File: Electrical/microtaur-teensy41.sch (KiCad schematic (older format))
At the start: 32 parts, among them J2 USB_A, U1 Teensy4.1, U3 LM7805_TO220

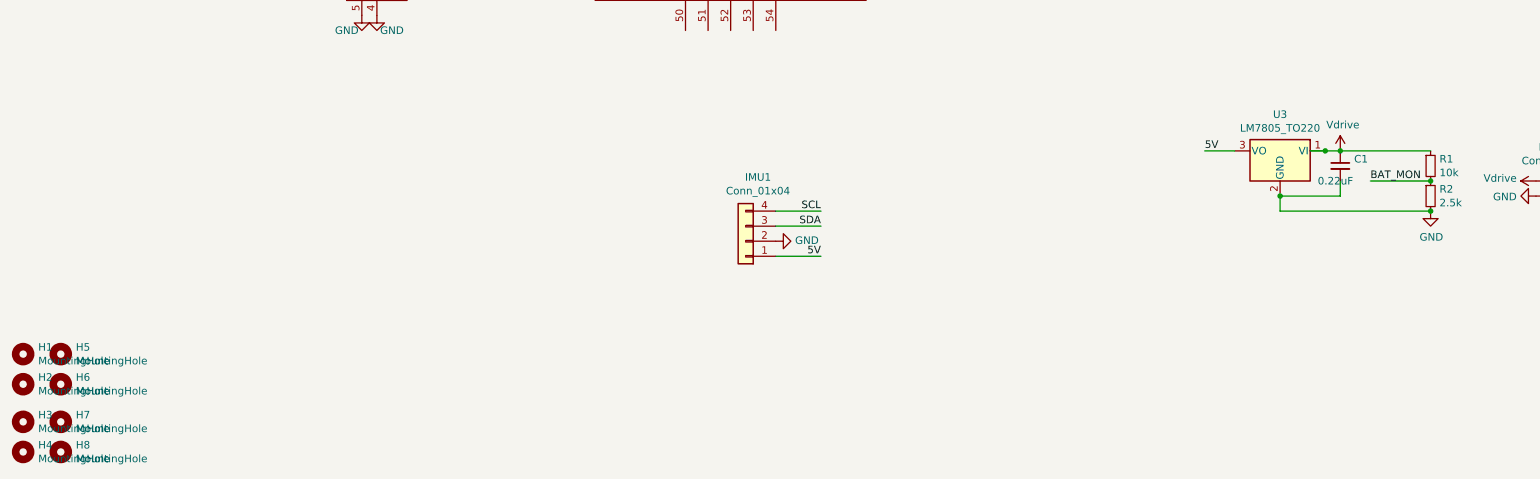
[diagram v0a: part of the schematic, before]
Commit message: completed pcb design, ready to fab
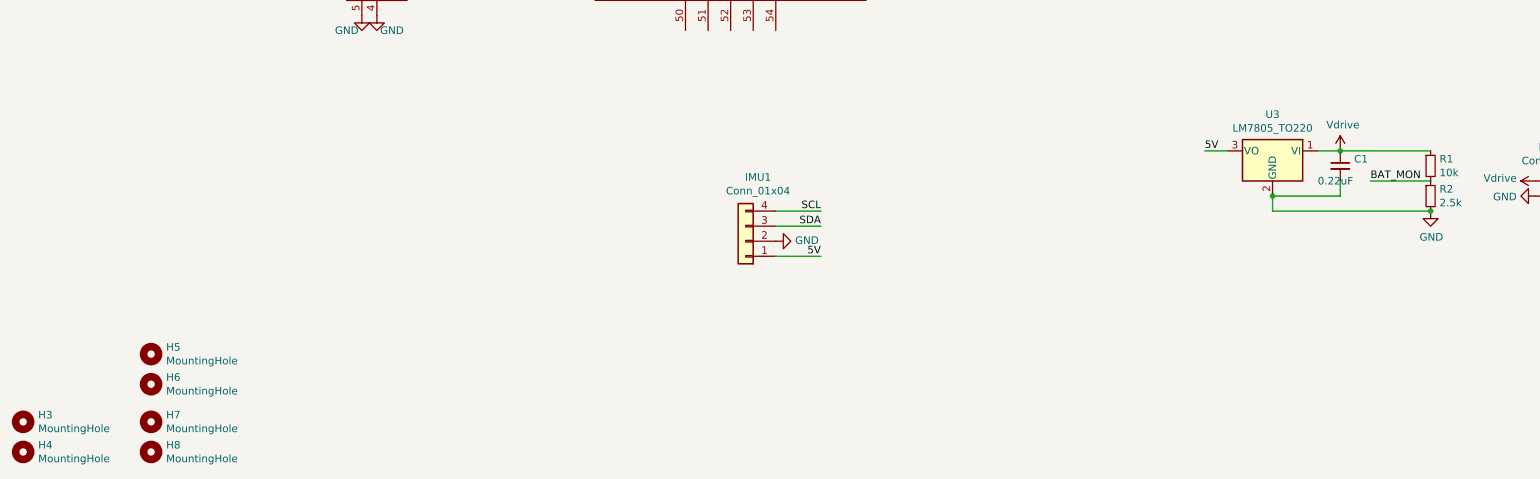
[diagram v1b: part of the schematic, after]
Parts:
- removed H1, H2: MountingHole, MountingHole:MountingHole_2.2mm_M2, symbol Mechanical:MountingHole
- IMU1: footprint Connector_JST:JST_SH_BM04B-SRSS-TB_1x04-1MP_P1.00mm_Vertical -> Connector_JST:JST_SH_SM04B-SRSS-TB_1x04-1MP_P1.00mm_Horizontal
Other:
- moved on the sheet: H5, H6, H7, H8, U3
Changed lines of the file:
@@
 Wire Wire Line
 	10100 5650 9700 5650
-Connection ~ 10100 5650
 Text Label 9700 5650 0    50   ~ 0
 BAT_MON
@@
 Text Label 6050 6150 2    50   ~ 0
 5V
-Connection ~ 9500 5450
 $Comp
 L Device:C_Small C1
@@
 $EndComp
 Wire Wire Line
-	9100 5750 9500 5750
+	9050 5750 9500 5750
 Wire Wire Line
 	9500 5750 9500 5650
 Wire Wire Line
-	9100 5850 9100 5750
-Wire Wire Line
-	9500 5450 10100 5450
-Wire Wire Line
-	9100 5850 10100 5850
-Connection ~ 10100 5850
-Wire Wire Line
-	8600 5450 8800 5450
+	9050 5850 9050 5750
+Wire Wire Line
+	9050 5850 10100 5850
 Text Label 8600 5450 0    50   ~ 0
 5V
@@
 L Mechanical:MountingHole H7
 U 1 1 608B8276
-P 1000 7250
-F 0 "H7" H 1100 7296 50  0000 L CNN
-F 1 "MountingHole" H 1100 7205 50  0000 L CNN
-F 2 "MountingHole:MountingHole_2.2mm_M2" H 1000 7250 50  0001 C CNN
-F 3 "~" H 1000 7250 50  0001 C CNN
-F 4 "~" H 1000 7250 50  0001 C CNN "Part Number"
-F 5 "~" H 1000 7250 50  0001 C CNN "URL"
-	1    1000 7250
+P 1600 7250
+F 0 "H7" H 1700 7296 50  0000 L CNN
+F 1 "MountingHole" H 1700 7205 50  0000 L CNN
+F 2 "MountingHole:MountingHole_2.2mm_M2" H 1600 7250 50  0001 C CNN
+F 3 "~" H 1600 7250 50  0001 C CNN
+F 4 "~" H 1600 7250 50  0001 C CNN "Part Number"
+F 5 "~" H 1600 7250 50  0001 C CNN "URL"
+	1    1600 7250
 	1    0    0    -1
 $EndComp
@@
 L Mechanical:MountingHole H8
 U 1 1 608B8652
-P 1000 7450
-F 0 "H8" H 1100 7496 50  0000 L CNN
-F 1 "MountingHole" H 1100 7405 50  0000 L CNN
-F 2 "MountingHole:MountingHole_2.2mm_M2" H 1000 7450 50  0001 C CNN
-F 3 "~" H 1000 7450 50  0001 C CNN
-F 4 "~" H 1000 7450 50  0001 C CNN "Part Number"
-F 5 "~" H 1000 7450 50  0001 C CNN "URL"
-	1    1000 7450
+P 1600 7450
+F 0 "H8" H 1700 7496 50  0000 L CNN
+F 1 "MountingHole" H 1700 7405 50  0000 L CNN
+F 2 "MountingHole:MountingHole_2.2mm_M2" H 1600 7450 50  0001 C CNN
+F 3 "~" H 1600 7450 50  0001 C CNN
+F 4 "~" H 1600 7450 50  0001 C CNN "Part Number"
+F 5 "~" H 1600 7450 50  0001 C CNN "URL"
+	1    1600 7450
 	1    0    0    -1
 $EndComp
@@
 $EndComp
 $Comp
-L Mechanical:MountingHole H2
-U 1 1 608B8C2F
-P 750 7000
-F 0 "H2" H 850 7046 50  0000 L CNN
-F 1 "MountingHole" H 850 6955 50  0000 L CNN
-F 2 "MountingHole:MountingHole_2.2mm_M2" H 750 7000 50  0001 C CNN
-F 3 "~" H 750 7000 50  0001 C CNN
-F 4 "~" H 750 7000 50  0001 C CNN "Part Number"
-F 5 "~" H 750 7000 50  0001 C CNN "URL"
-	1    750  7000
-	1    0    0    -1
-$EndComp
-$Comp
 L Mechanical:MountingHole H6
 U 1 1 608B8EC9
-P 1000 7000
-F 0 "H6" H 1100 7046 50  0000 L CNN
-F 1 "MountingHole" H 1100 6955 50  0000 L CNN
-F 2 "MountingHole:MountingHole_2.2mm_M2" H 1000 7000 50  0001 C CNN
-F 3 "~" H 1000 7000 50  0001 C CNN
-F 4 "~" H 1000 7000 50  0001 C CNN "Part Number"
-F 5 "~" H 1000 7000 50  0001 C CNN "URL"
-	1    1000 7000
+P 1600 7000
+F 0 "H6" H 1700 7046 50  0000 L CNN
+F 1 "MountingHole" H 1700 6955 50  0000 L CNN
+F 2 "MountingHole:MountingHole_2.2mm_M2" H 1600 7000 50  0001 C CNN
+F 3 "~" H 1600 7000 50  0001 C CNN
+F 4 "~" H 1600 7000 50  0001 C CNN "Part Number"
+F 5 "~" H 1600 7000 50  0001 C CNN "URL"
+	1    1600 7000
 	1    0    0    -1
 $EndComp
@@
 L Mechanical:MountingHole H5
 U 1 1 608B9277
-P 1000 6800
-F 0 "H5" H 1100 6846 50  0000 L CNN
-F 1 "MountingHole" H 1100 6755 50  0000 L CNN
-F 2 "MountingHole:MountingHole_2.2mm_M2" H 1000 6800 50  0001 C CNN
-F 3 "~" H 1000 6800 50  0001 C CNN
-F 4 "~" H 1000 6800 50  0001 C CNN "Part Number"
-F 5 "~" H 1000 6800 50  0001 C CNN "URL"
-	1    1000 6800
-	1    0    0    -1
-$EndComp
-$Comp
-L Mechanical:MountingHole H1
-U 1 1 608B9565
-P 750 6800
-F 0 "H1" H 850 6846 50  0000 L CNN
-F 1 "MountingHole" H 850 6755 50  0000 L CNN
-F 2 "MountingHole:MountingHole_2.2mm_M2" H 750 6800 50  0001 C CNN
-F 3 "~" H 750 6800 50  0001 C CNN
-F 4 "~" H 750 6800 50  0001 C CNN "Part Number"
-F 5 "~" H 750 6800 50  0001 C CNN "URL"
-	1    750  6800
+P 1600 6800
+F 0 "H5" H 1700 6846 50  0000 L CNN
+F 1 "MountingHole" H 1700 6755 50  0000 L CNN
+F 2 "MountingHole:MountingHole_2.2mm_M2" H 1600 6800 50  0001 C CNN
+F 3 "~" H 1600 6800 50  0001 C CNN
+F 4 "~" H 1600 6800 50  0001 C CNN "Part Number"
+F 5 "~" H 1600 6800 50  0001 C CNN "URL"
+	1    1600 6800
 	1    0    0    -1
 $EndComp
@@
 F 0 "IMU1" H 5468 5625 50  0000 C CNN
 F 1 "Conn_01x04" H 5468 5716 50  0000 C CNN
-F 2 "Connector_JST:JST_SH_BM04B-SRSS-TB_1x04-1MP_P1.00mm_Vertical" H 5550 6050 50  0001 C CNN
+F 2 "Connector_JST:JST_SH_SM04B-SRSS-TB_1x04-1MP_P1.00mm_Horizontal" H 5550 6050 50  0001 C CNN
 F 3 "~" H 5550 6050 50  0001 C CNN
 F 4 "455-1790-2-ND" H 5550 6050 50  0001 C CNN "Part Number"
@@
 	-1   0    0    1
 $EndComp
-Connection ~ 9100 5750
-Wire Wire Line
-	9400 5450 9500 5450
-Wire Wire Line
-	9300 5450 9400 5450
-Connection ~ 9400 5450
 $Comp
 L Regulator_Linear:LM7805_TO220 U3
 U 1 1 6097103B
-P 9100 5450
-F 0 "U3" H 9100 5692 50  0000 C CNN
-F 1 "LM7805_TO220" H 9100 5601 50  0000 C CNN
-F 2 "Package_TO_SOT_SMD:SOT-223" H 9100 5675 50  0001 C CIN
-F 3 "" H 9100 5400 50  0001 C CNN
-F 4 "NCP1117LPST33T3COSTR-ND" H 9100 5450 50  0001 C CNN "Part Number"
-F 5 "https://www.digikey.com/en/products/detail/on-semiconductor/NCP1117LPST33T3G/2194024" H 9100 5450 50  0001 C CNN "URL"
-	1    9100 5450
+P 9050 5450
+F 0 "U3" H 9050 5692 50  0000 C CNN
+F 1 "LM7805_TO220" H 9050 5601 50  0000 C CNN
+F 2 "Package_TO_SOT_SMD:SOT-223" H 9050 5675 50  0001 C CIN
+F 3 "" H 9050 5400 50  0001 C CNN
+F 4 "NCP1117LPST33T3COSTR-ND" H 9050 5450 50  0001 C CNN "Part Number"
+F 5 "https://www.digikey.com/en/products/detail/on-semiconductor/NCP1117LPST33T3G/2194024" H 9050 5450 50  0001 C CNN "URL"
+	1    9050 5450
 	-1   0    0    -1
 $EndComp
+Connection ~ 9500 5450
+Wire Wire Line
+	9500 5450 10100 5450
+Wire Wire Line
+	9350 5450 9500 5450
+Wire Wire Line
+	8600 5450 8750 5450
+Connection ~ 10100 5850
+Connection ~ 9050 5750
 $EndSCHEMATC
